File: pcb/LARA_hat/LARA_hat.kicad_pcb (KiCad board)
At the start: 2 copper layers, 65 x 56 mm, 33 parts, among them J1 Raspberry_Pi_4, J2 Conn_RoboClaw, J3 Conn_Dynamixel, J4 Conn_01x02_Pin, J5 12V in, J6 LED_JST, J7 I2C_JST, U1 MCP2515-xSO, U2 SN65HVD230, U3 74LVC2G241, U4 Buck 12V - 5V, Y1 8MHz

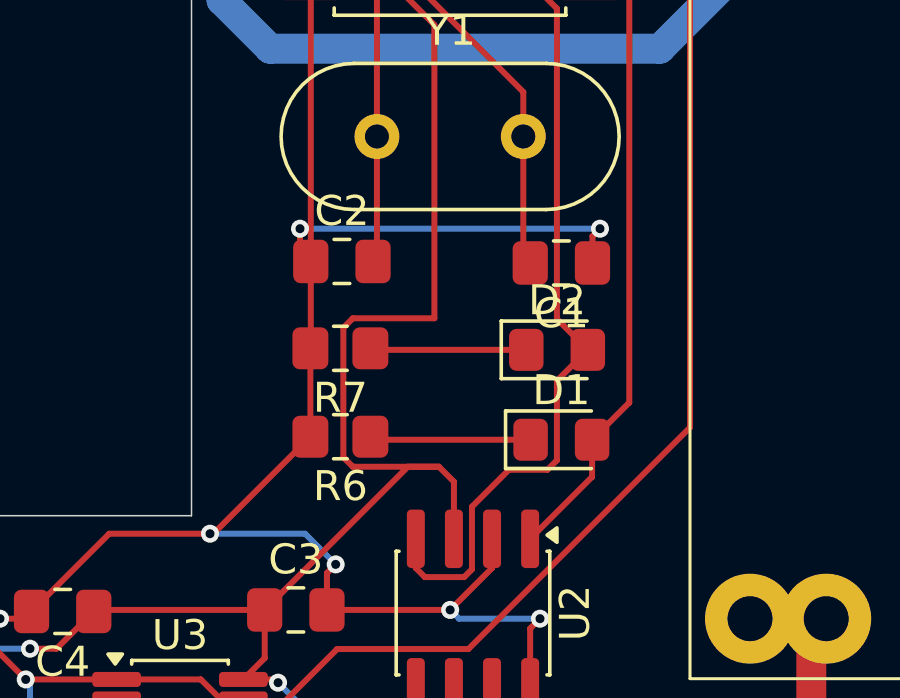
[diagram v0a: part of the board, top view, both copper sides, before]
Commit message: pcb
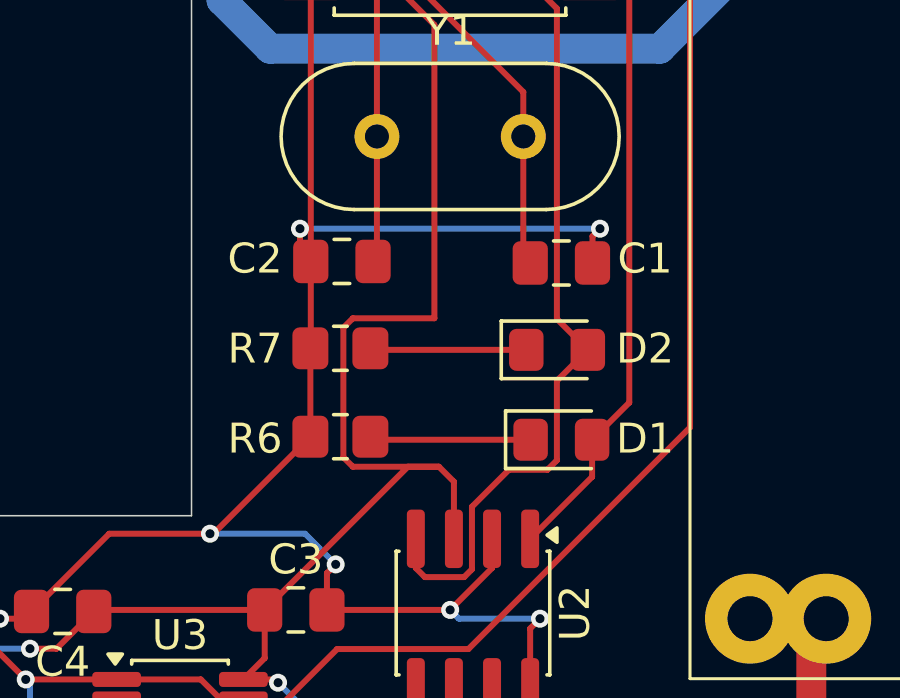
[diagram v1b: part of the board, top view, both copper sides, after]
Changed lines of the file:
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@@
 		(tenting front back)
 		(pcbplotparams
-			(layerselection 0x00000000_00000000_55555555_575555ff)
+			(layerselection 0x00000000_00000000_55555555_5755f5ff)
 			(plot_on_all_layers_selection 0x00000000_00000000_00000000_00000000)
 			(disableapertmacros no)
-			(usegerberextensions no)
+			(usegerberextensions yes)
 			(usegerberattributes yes)
 			(usegerberadvancedattributes yes)
-			(creategerberjobfile yes)
+			(creategerberjobfile no)
 			(dashed_line_dash_ratio 12.000000)
 			(dashed_line_gap_ratio 3.000000)
@@
 		(tags "LED handsolder")
 		(property "Reference" "D1"
-			(at 0 -1.65 0)
+			(at 2.7876 -0.0356 0)
 			(layer "F.SilkS")
 			(effects
@@
 		(tags "capacitor handsolder")
 		(property "Reference" "C2"
-			(at 0 -1.68 0)
+			(at -2.8972 -0.092 0)
 			(layer "F.SilkS")
 			(effects
@@
 		(tags "LED handsolder")
 		(property "Reference" "D2"
-			(at 0 -1.65 0)
+			(at 2.931 -0.0384 0)
 			(layer "F.SilkS")
 			(effects
@@
 		(tags "resistor handsolder")
 		(property "Reference" "R7"
-			(at 0 -1.65 0)
+			(at 2.8464 -0.0124 0)
 			(layer "F.SilkS")
 			(effects
@@
 		(tags "capacitor handsolder")
 		(property "Reference" "C1"
-			(at 0 -1.68 0)
+			(at -2.7876 0.1428 0)
 			(layer "F.SilkS")
 			(effects
@@
 		(tags "resistor handsolder")
 		(property "Reference" "R6"
-			(at 0 -1.65 0)
+			(at 2.8464 -0.066 0)
 			(layer "F.SilkS")
 			(effects
